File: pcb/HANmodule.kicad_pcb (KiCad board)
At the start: 2 copper layers, 62 x 46 mm, 32 parts, among them J1 HAN port, J2 Debug, J3 Prog, SW1 Reset, U1 RT9013-3.3v, U2 ESP-12F

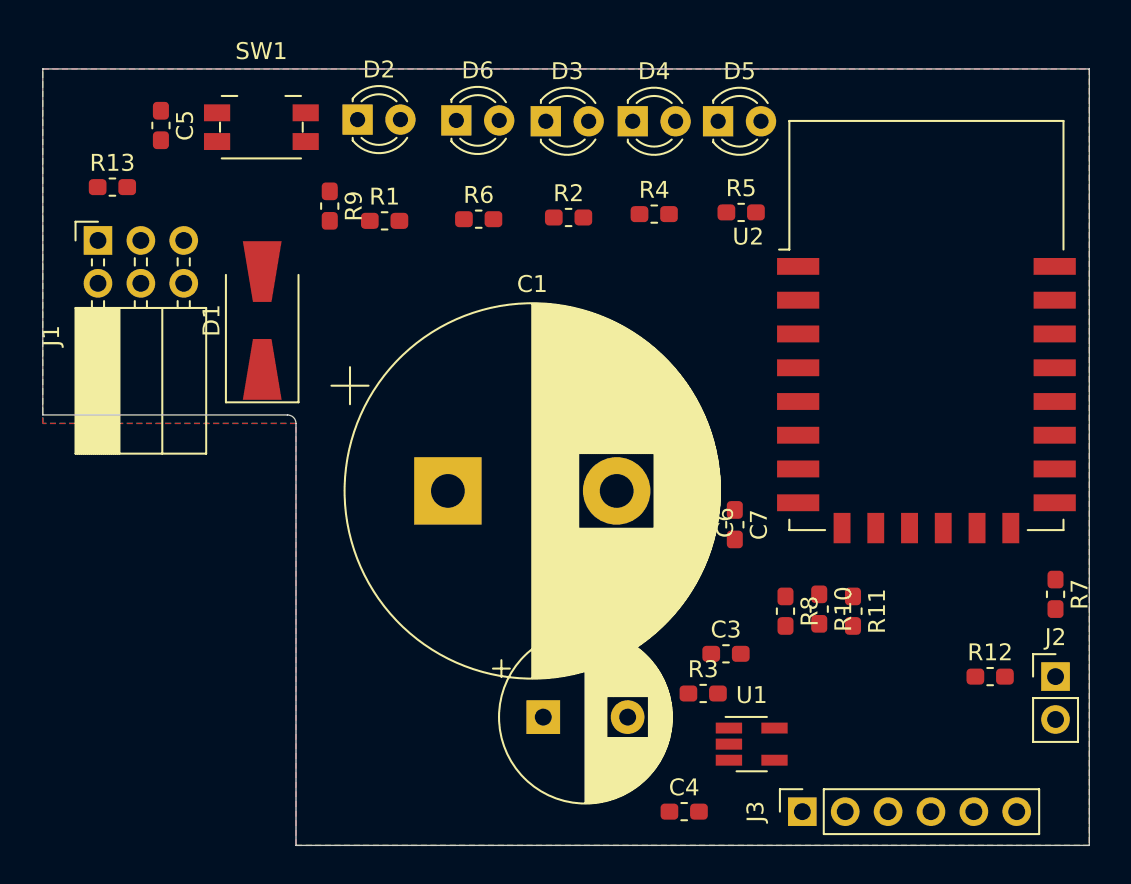
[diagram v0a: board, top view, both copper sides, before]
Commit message: PCB rev 1
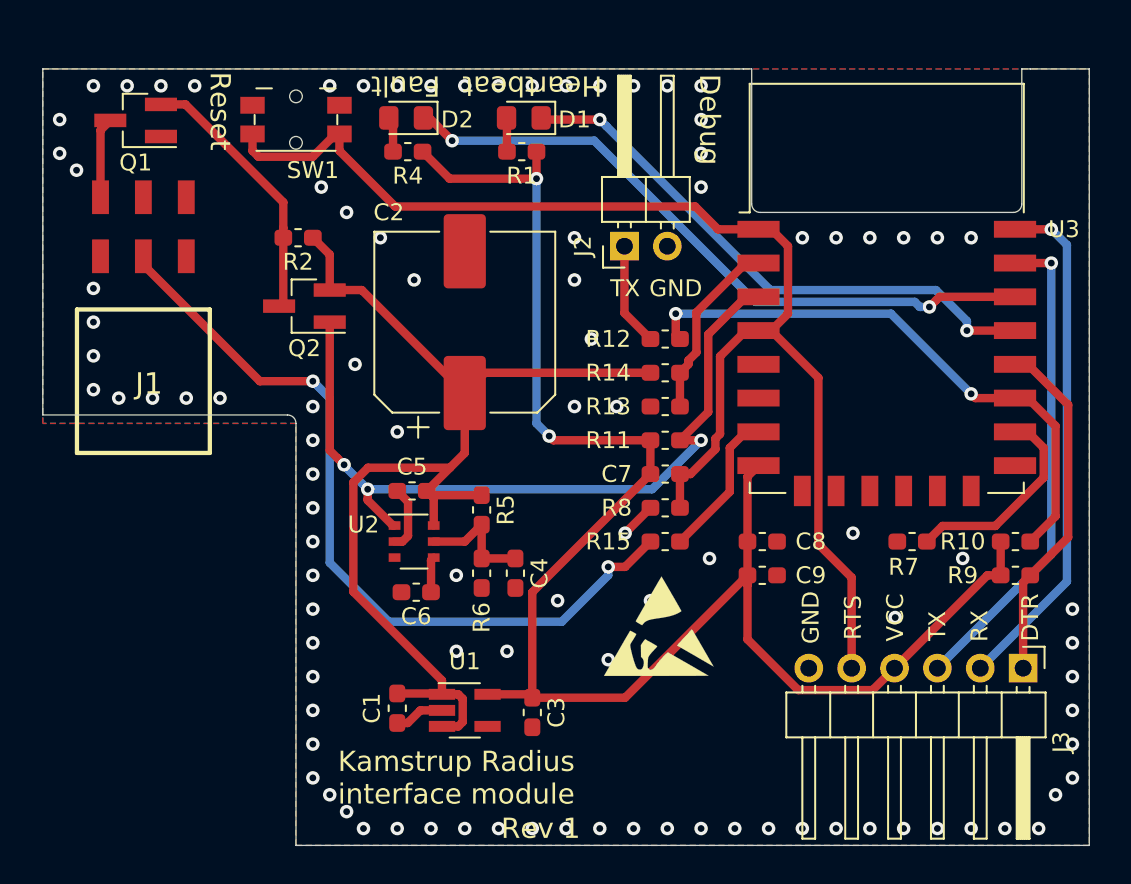
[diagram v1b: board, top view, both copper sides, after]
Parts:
- removed D3: Meter data, LED_THT:LED_D3.0mm
- removed D4: Wifi, LED_THT:LED_D3.0mm
- removed D5: MQTT, LED_THT:LED_D3.0mm
- removed D6: Fault, LED_THT:LED_D3.0mm
- removed R3: 100k, Resistor_SMD:R_0603_1608Metric_Pad1.05x0.95mm_HandSolder
- added C8: 10uF, Capacitor_SMD:C_0603_1608Metric_Pad1.05x0.95mm_HandSolder, F.Cu at (137.6, 73.0)
- added C9: 100n, Capacitor_SMD:C_0603_1608Metric_Pad1.05x0.95mm_HandSolder, F.Cu at (137.6, 75.0)
- added Q1: SI2301DS_P-FET, Package_TO_SOT_SMD:SOT-23_Handsoldering, F.Cu at (100.5, 48.0)
- added Q2: BSS139, Package_TO_SOT_SMD:SOT-23_Handsoldering, F.Cu at (110.5, 59.0)
- added R14: 34k, Resistor_SMD:R_0603_1608Metric_Pad1.05x0.95mm_HandSolder, F.Cu at (131.9, 65.0)
- added R15: 100k, Resistor_SMD:R_0603_1608Metric_Pad1.05x0.95mm_HandSolder, F.Cu at (131.9, 73.0)
- added REF**: ESD-Logo_6.6x6mm_SilkScreen, Symbol:ESD-Logo_6.6x6mm_SilkScreen, B.Cu at (145.5, 60.5)
- added REF**: ESD-Logo_6.6x6mm_SilkScreen, Symbol:ESD-Logo_6.6x6mm_SilkScreen, F.Cu at (131.5, 78.0)
- added U3: ESP-12F, RF_Module:ESP-12E, F.Cu at (145.0, 58.0)
- C1: value CP -> 1uF; footprint Capacitor_THT:CP_Radial_D22.0mm_P10.00mm_SnapIn -> Capacitor_SMD:C_0603_1608Metric_Pad1.05x0.95mm_HandSolder
- C2: value CP -> 0.1F 5.5V FC0H104ZFTBR24; footprint Capacitor_THT:CP_Radial_D10.0mm_P5.00mm -> Capacitor_SMD:CP_Elec_10x10.5
- C4: value 1uF -> 1n
- C6: value 10uF -> 1,75u
- D1: value D_Schottky -> Heartbeat; footprint Diode_SMD:D_SMA-SMB_Universal_Handsoldering -> LED_SMD:LED_0805_2012Metric_Pad1.15x1.40mm_HandSolder
- D2: value Heartbeat -> Fault; footprint LED_THT:LED_D3.0mm -> LED_SMD:LED_0805_2012Metric_Pad1.15x1.40mm_HandSolder
- J1: value HAN port -> M20-7920342R; footprint Connector_PinSocket_2.54mm:PinSocket_2x03_P2.54mm_Horizontal -> SamacSys_Parts:M20-7920342R
- J2: footprint Connector_PinHeader_2.54mm:PinHeader_1x02_P2.54mm_Vertical -> Connector_PinHeader_2.54mm:PinHeader_1x02_P2.54mm_Horizontal
- J3: footprint Connector_PinSocket_2.54mm:PinSocket_1x06_P2.54mm_Vertical -> Connector_PinHeader_2.54mm:PinHeader_1x06_P2.54mm_Horizontal
- R12: value 1k -> 100k
- R13: value 1k -> 102k
- R2: value 1k -> 55R
- R5: value 1k -> 113k
- R6: value 1k -> 13k3
- SW1: footprint Button_Switch_SMD:Panasonic_EVQPUJ_EVQPUA -> Button_Switch_SMD:Panasonic_EVQPUM_EVQPUD
- U1: value RT9013-3.3v -> TLV75530PDBV | RT9013
- U2: value ESP-12F -> NCP308SNADJT1G; footprint RF_Module:ESP-12E -> Package_SO:TSOP-6_1.65x3.05mm_P0.95mm
- moved R9 46.1 mm to (152.6, 75.0), turned to 180 degrees
- moved J2 36.1 mm to (129.5, 55.5), turned to 90 degrees
- moved R13 34.5 mm to (131.9, 63.0), turned to 180 degrees
- moved U2 32.9 mm to (117.0, 73.0)
- moved R12 27.8 mm to (131.9, 61.0), turned to 180 degrees
- moved C5 26.3 mm to (116.9, 70.0), turned to 0 degrees
- moved C2 23.9 mm to (120.0, 60.0), turned to 90 degrees
- moved R5 23.4 mm to (121.0, 71.1), turned to 270 degrees
- moved R6 21.0 mm to (121.0, 74.9), turned to 270 degrees
- moved D1 19.6 mm to (123.5, 47.9), turned to 180 degrees
- moved C6 17.4 mm to (117.1, 76.0), turned to 180 degrees
- moved C4 17.3 mm to (123.0, 74.9), turned to 270 degrees
- moved U1 17.1 mm to (120.0, 83.0)
- moved R2 16.1 mm to (110.1, 55.0), turned to 180 degrees
- moved J3 15.6 mm to (153.1, 80.5), turned to 270 degrees
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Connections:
- C1 pad 1: Net-(C1-Pad1) -> +4V
- C1 pad 2: Net-(C1-Pad2) -> GND
- C2 pad 1: Net-(C1-Pad2) -> +4V
- C3 pad 1: Net-(C1-Pad1) -> +3V0
- C4 pad 1: +3V3 -> Net-(C4-Pad1)
- C5 pad 2: /~RST -> +4V
- C6 pad 1: +3V3 -> Net-(C6-Pad1)
- C7 pad 1: +3V3 -> GND
- C7 pad 2: GND -> /~RST
- D1 pad 1: Net-(C1-Pad1) -> /~LED
- D1 pad 2: VCC -> Net-(D1-Pad2)
- D2 pad 1: /GPIO0 -> /~FAULT_LED
- J1 pad 1: Net-(J1-Pad1) -> (no net)
- J1 pad 2: /DIN -> (no net)
- J1 pad 3: VCC -> (no net)
- J1 pad 4: GND -> /DOUT
- J1 pad 5: /DOUT -> VCC
- J1 pad 6: Net-(J1-Pad6) -> GND
- J3 pad 1: Net-(J3-Pad1) -> /GPIO0
- J3 pad 2: Net-(J3-Pad2) -> /TX
- J3 pad 3: Net-(J3-Pad3) -> /RX
- J3 pad 4: Net-(J3-Pad4) -> +3V0
- J3 pad 5: Net-(J3-Pad5) -> /~RST
- J3 pad 6: Net-(J3-Pad6) -> GND
- R1 pad 1: +3V3 -> +3V0
- R1 pad 2: Net-(D2-Pad2) -> Net-(D1-Pad2)
- R10 pad 1: /GPIO0 -> /GPIO2
- R10 pad 2: +3V3 -> +3V0
- R11 pad 1: /GPIO2 -> +3V0
- R11 pad 2: +3V3 -> /EN
- R13 pad 1: /DIN -> Net-(R13-Pad1)
- R13 pad 2: Net-(R13-Pad2) -> +4V
- R2 pad 1: +3V3 -> +4V
- R4 pad 1: +3V3 -> +3V0
- R4 pad 2: Net-(D4-Pad2) -> Net-(D2-Pad2)
- R5 pad 1: +3V3 -> +4V
- R5 pad 2: Net-(D5-Pad2) -> Net-(C4-Pad1)
- R6 pad 1: +3V3 -> Net-(C4-Pad1)
- R6 pad 2: Net-(D6-Pad2) -> GND
- R8 pad 1: /EN -> /~RST
- R8 pad 2: +3V3 -> +3V0
- R9 pad 1: /~RST -> /GPIO0
- R9 pad 2: +3V3 -> +3V0
- U1 pad 1: Net-(C1-Pad1) -> +4V
- U1 pad 3: Net-(C1-Pad1) -> +4V
- U1 pad 4: Net-(U1-Pad4) -> (no net)
- U1 pad 5: +3V3 -> +3V0
- U2 pad 1: /RST -> /EN
- U2 pad 2: Net-(U2-Pad2) -> GND
- U2 pad 3: /EN -> (no net)
- U2 pad 4: Net-(U2-Pad4) -> Net-(C6-Pad1)
- U2 pad 5: /FAULT_LED -> Net-(C4-Pad1)
- U2 pad 6: /MQTT_LED -> +4V
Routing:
- net +3V0: track 0.00 -> 98.9 mm, vias 0 -> 2
- net /~RST: track 0.00 -> 78.1 mm
- net +4V: track 0.00 -> 65.4 mm
- net /DOUT: track 0.00 -> 47.3 mm, vias 0 -> 2
- net /EN: track 0.00 -> 46.8 mm, vias 0 -> 3
- net /~FAULT_LED: track 0.00 -> 39.9 mm, vias 0 -> 2
- net /GPIO2: track 0.00 -> 34.3 mm, vias 0 -> 2
- net /~LED: track 0.00 -> 33.6 mm, vias 0 -> 2
- net /TX: track 0.00 -> 30.7 mm, vias 0 -> 1
- net /RX: track 0.00 -> 28.9 mm, vias 0 -> 1
- net /GPIO0: track 0.00 -> 20.9 mm
- net Net-(Q1-Pad2): track 0.00 -> 15.9 mm
- net /GPIO15: track 0.00 -> 12.3 mm
- net Net-(R13-Pad1): track 0.00 -> 10.9 mm
- net GND: track 0.00 -> 8.95 mm, vias 0 -> 100
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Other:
- outline, holes or cut-outs redrawn
- rule trace_min: 0.2 -> 0.14
- board text added: "DTR"
- board text added: "Debug"
- board text added: "Fault"
- board text added: "GND"
- board text added: "Heartbeat"
- board text added: "Kamstrup Radius interface module"
- board text added: "RTS"
- board text added: "RX"
- board text added: "Reset"
- board text added: "Rev 1"
- board text added: "TX"
- board text added: "VCC"
- board text added: "https://github.com/Asbjoern /Kamstrup-Radius-Interface"
